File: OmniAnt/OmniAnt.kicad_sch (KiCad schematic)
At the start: 14 parts, among them J1 Conn_01x02_Pin, J2 USB_B_Micro, J3 Connector, USB-TYPE-C-16P, U1 ESP32-S3-WROOM-1, U2 TPSM53603RDA, U4 USBLC6-2P6

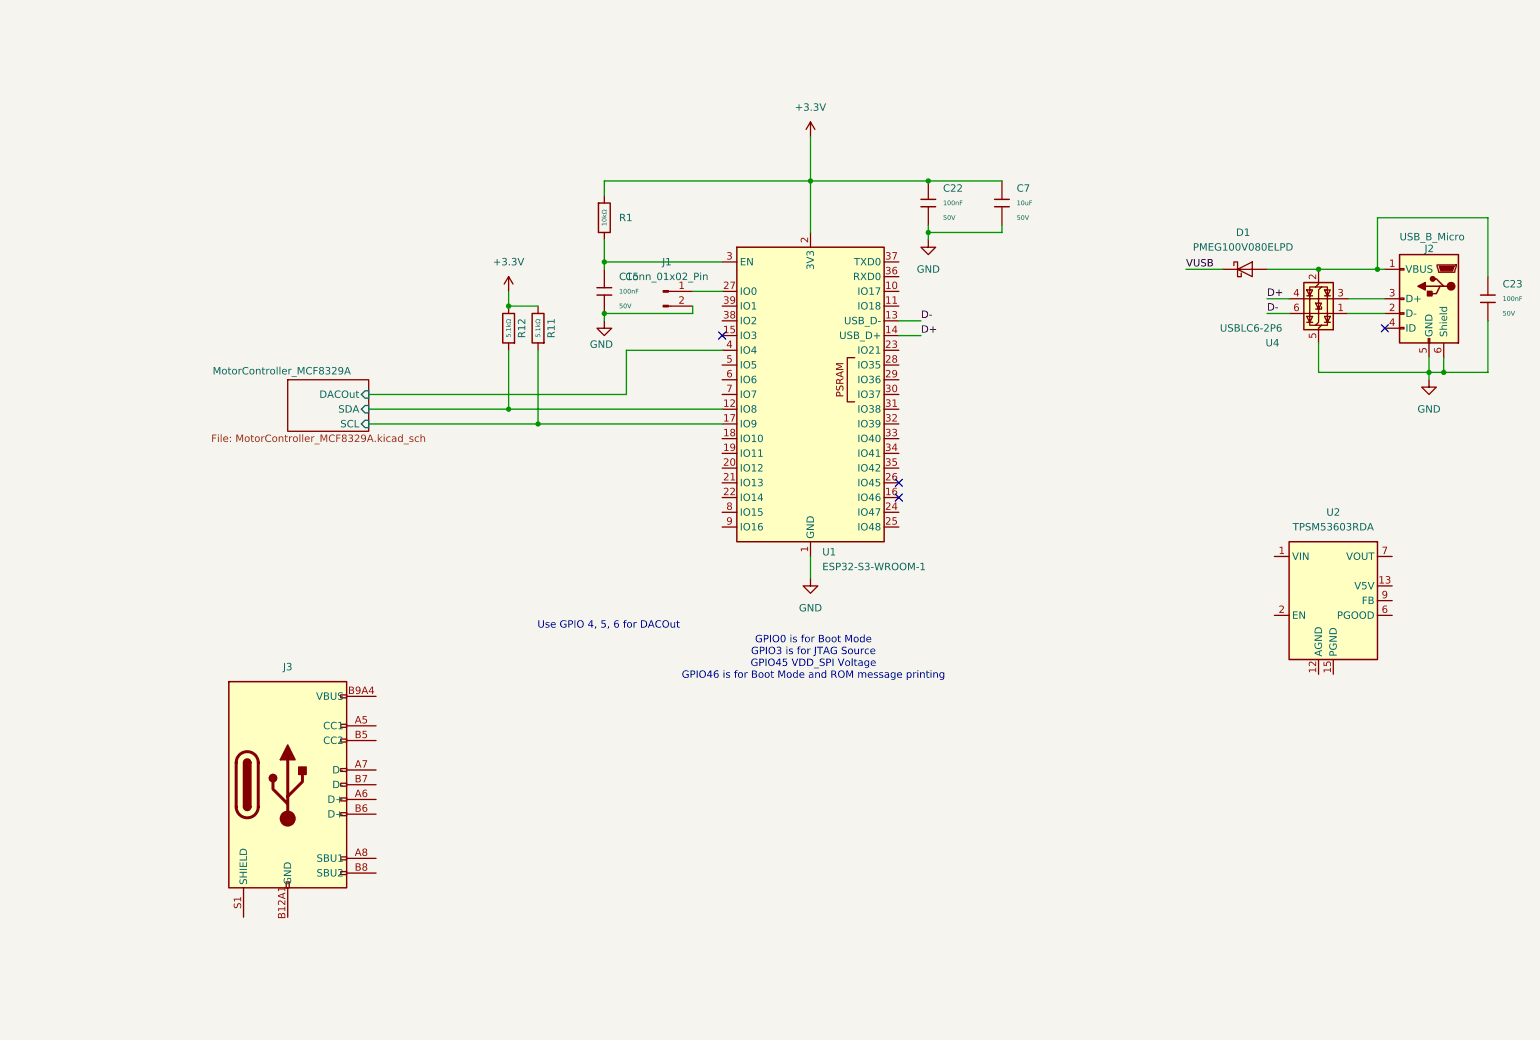
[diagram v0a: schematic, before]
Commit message: Good progress on the power stage today.
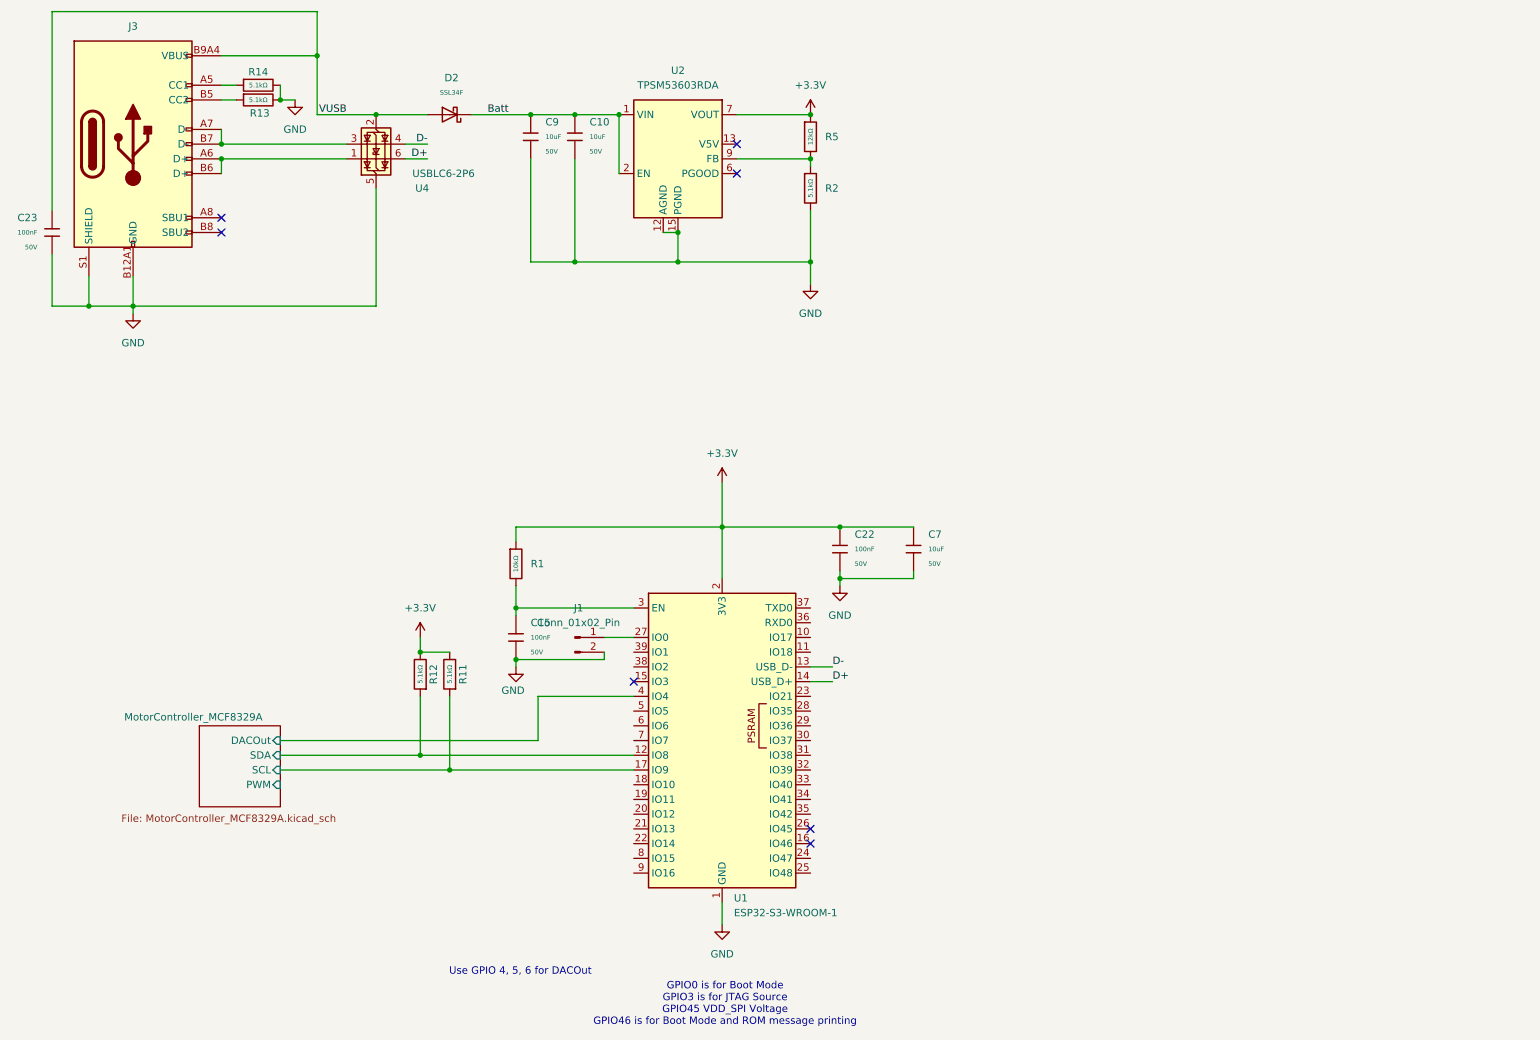
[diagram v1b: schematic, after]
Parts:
- removed D1: PMEG100V080ELPD, Package_TO_SOT_SMD:Nexperia_CFP15_SOT-1289, symbol Diode:PMEG100V080ELPD
- removed J2: USB_B_Micro, symbol Connector:USB_B_Micro
- added C10, C9: 10uF, PCM_JLCPCB:C_0805, symbol PCM_JLCPCB-Capacitors:0805,10uF,(2)
- added D2: SSL34F, PCM_JLCPCB:D_SMAF, symbol PCM_JLCPCB-Diodes:Schottky,SSL34F
- added R13, R14, R2: 5.1kΩ, PCM_JLCPCB:R_0402, symbol PCM_JLCPCB-Resistors:0402,5.1kΩ
- added R5: 12kΩ, PCM_JLCPCB:R_0402, symbol PCM_JLCPCB-Resistors:0402,12kΩ
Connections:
- net +3.3V: now also U2.7 (VOUT), U2.8 (VOUT), R5.1
- net D+: now also U4.6 (I/O1); no longer U4.4 (I/O2)
- net D-: now also U4.4 (I/O2); no longer U4.6 (I/O1)
- net GND: now also J3.A12B1 (GND), J3.B12A1 (GND), J3.S1 (SHIELD), U2.10 (PGND), U2.11 (PGND), U2.12 (AGND), U2.15 (PGND), U2.3 (PGND), C10.2, C9.2, R13.2, R14.2, R2.2
- net VUSB: now also C23.1, J3.A9B4 (VBUS), J3.B9A4 (VBUS), U4.2 (GND), D2.2
- net at J3.A5 (CC1): now also R14.1
- net at J3.A6 (D+): now also J3.B6 (D+), U4.1 (I/O1)
- net at J3.A7 (D-): now also J3.B7 (D-), U4.3 (I/O2)
- net at J3.B5 (CC2): now also R13.1
- net Batt: now reaches U2.1 (VIN), U2.14 (VIN)
- net Batt: now also U2.2 (EN), C10.1, C9.1, D2.1
- net at U2.9 (FB): now also R2.1, R5.2
- no-connect marks 4 -> 7
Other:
- sheet MotorController_MCF8329A ports: added PWM; removed none
- moved on the sheet: C15, C22, C23, C7, J1, J3, R1, R11, R12, U1, U2, U4
